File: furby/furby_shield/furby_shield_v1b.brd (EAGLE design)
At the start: 68.6 x 53.3 mm, 26 parts, among them IC1 UA7805CKCS, Q2 ZVNL110ASTZ, Q3 ZVNL110ASTZ

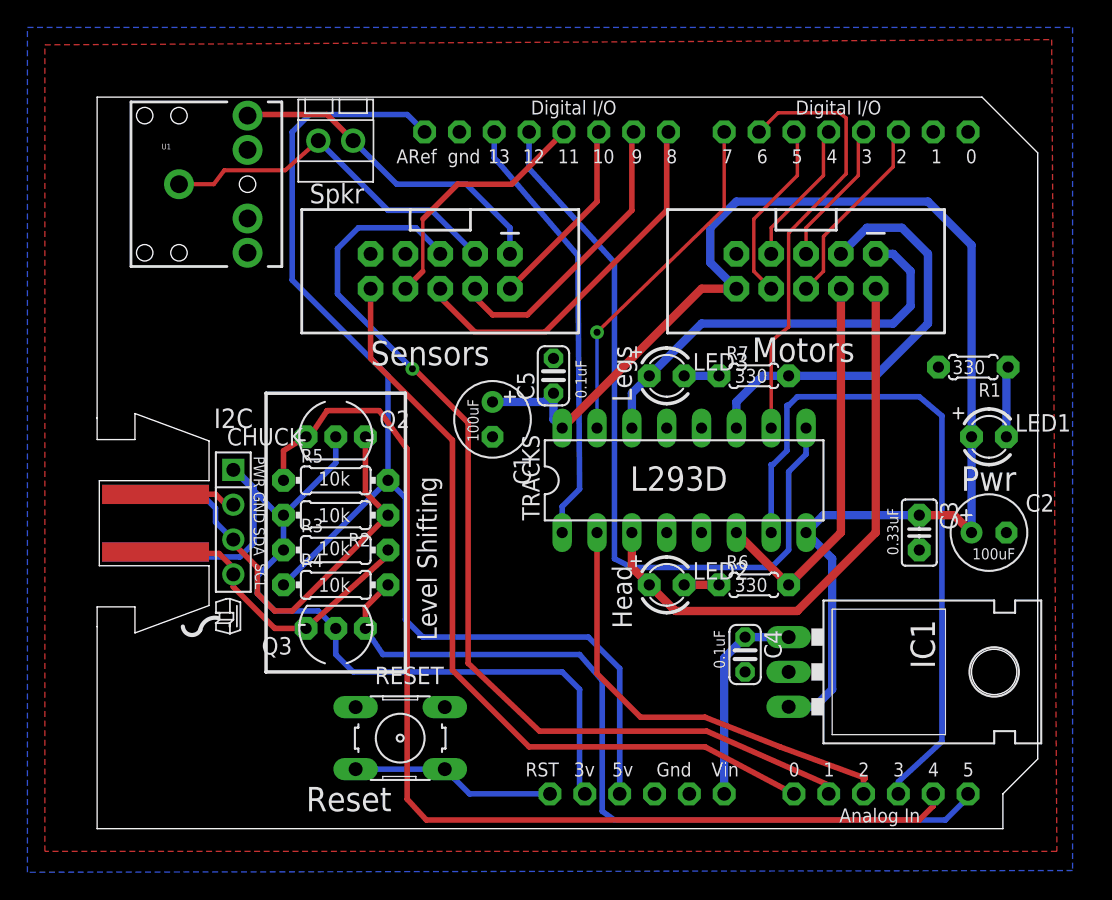
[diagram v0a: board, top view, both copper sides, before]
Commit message: furby updates
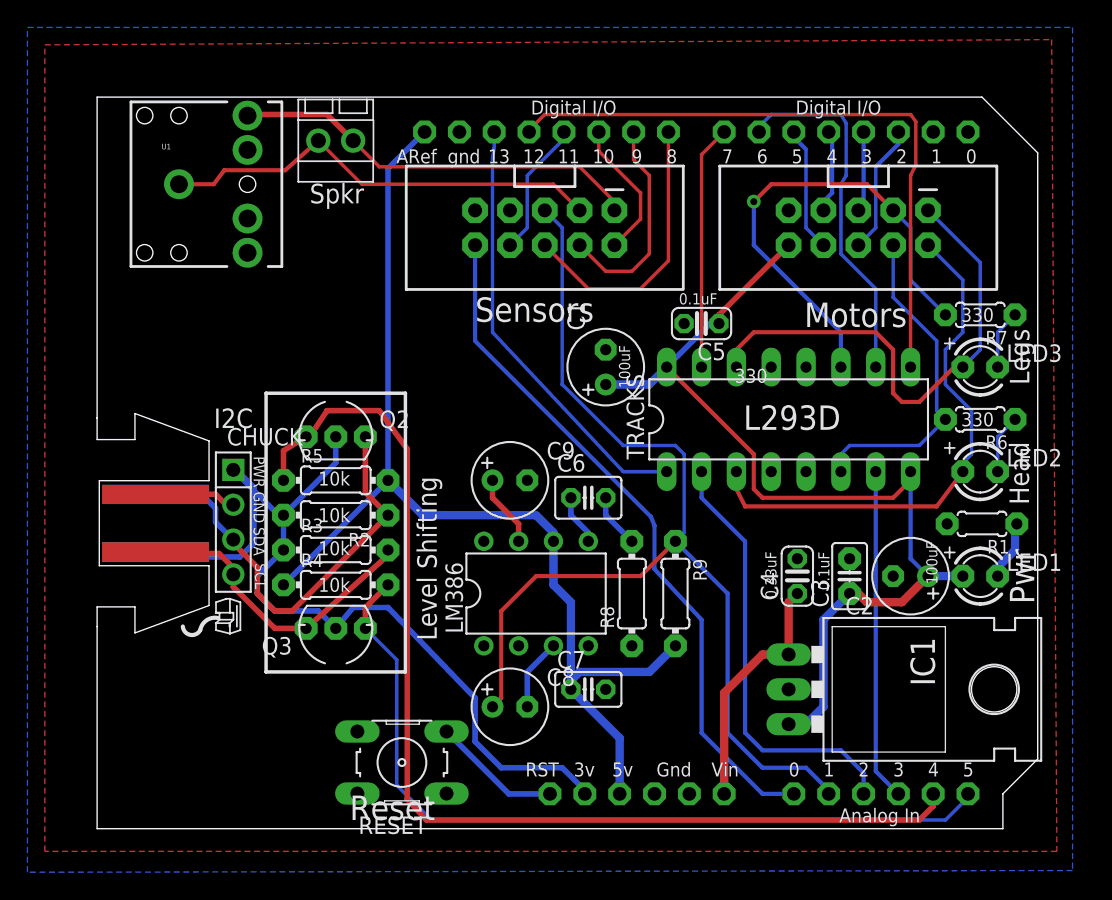
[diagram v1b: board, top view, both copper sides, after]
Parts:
- added C6: 47nF, rcl:C025-030X050
- added C7: 100nF, rcl:C025-025X050
- added C8, C9: 10uF, rcl:E2,5-6
- added LM386: (no value), linear:DIL08
- added R8, R9: (no value), adafruit:0204/7
- moved LED2 24.3 mm to (64.8, 26.0)
- moved LED3 22.9 mm to (64.8, 33.7)
- moved R6 20.4 mm to (64.8, 29.8), turned to 180 degrees
- moved R7 17.1 mm to (64.8, 37.5), turned to 180 degrees
- moved C5 11.4 mm to (44.5, 36.8), turned to 180 degrees
- moved R1 11.4 mm to (64.9, 22.2)
- moved LED1 10.2 mm to (64.8, 18.4)
- moved C1 9.09 mm to (37.5, 33.7), turned to 90 degrees
- moved TRACKS 8.82 mm to (50.8, 29.8)
- moved SENSORS 8.26 mm to (33.0, 43.8)
- moved C4 6.87 mm to (51.4, 18.4), turned to 90 degrees
- moved C2 6.54 mm to (59.7, 18.4), turned to 180 degrees
- moved C3 5.99 mm to (55.2, 18.4), turned to 90 degrees
- moved MOTORS 4.96 mm to (55.9, 43.8)
- moved RESET 1.78 mm to (22.6, 4.83), turned to 180 degrees
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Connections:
- removed net MIC_B: SENSORS.7
- new net A1: C6.1, LM386.5
- new net N$4: C6.2, R8.2
- new net N$6: C9.+, LM386.7
- new net N$8: C8.-, LM386.3
- net GND: now also C7.2, C9.-, LM386.2, LM386.4, R8.1; no longer RESET.2
- net MIC_A: now also C8.+, R9.1
- net RESET: no longer RESET.4
- net VCC: now also C7.1, LM386.6, R9.2
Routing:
- net +5V: track 100.8 -> 71.9 mm
- net UM1: track 50.8 -> 24.2 mm
- net D12: track 56.3 -> 47.0 mm
- net PIEZO: track 18.5 -> 9.89 mm
- net LM2: track 25.5 -> 17.8 mm, vias 1 -> 0
- net LEVEL_A: track 58.3 -> 50.8 mm
- net BEAK: track 27.6 -> 20.6 mm
- net SPR_B: track 26.3 -> 32.6 mm
- net L_MTR_1: track 31.1 -> 36.9 mm
- net BELLY: track 21.5 -> 15.8 mm
- net LM1: track 32.0 -> 26.4 mm
- net SPR_A: track 24.5 -> 30.0 mm
- net RESET: track 14.9 -> 9.43 mm
- net VCC: track 86.7 -> 81.3 mm
- net N$8: track 0.00 -> 5.23 mm
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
